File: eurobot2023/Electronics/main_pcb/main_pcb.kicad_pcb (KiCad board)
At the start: 2 copper layers, 103.1 x 93.2 mm, 51 parts, among them IC1 CD74HCT125M96, IC2 SN74LVC126ADR, J1 PI40HAT, J10 Conn_01x02_Male, J11 MagneticEncoder, J12 Conn_01x07_Male, J13 MagneticEncoder, J14 Conn_01x03_Male, J15 Conn_01x02_Male, J16 Conn_01x02_Male, J17 Conn_01x02_Male, J18 Conn_01x02_Male, J19 Conn_01x02_Male, J2 Conn_01x02_Male, J20 Conn_01x03_Male, J21 Conn_01x03_Male, J22 Conn_01x02_Male, J23 Conn_01x02_Male, J24 Conn_01x03_Male, J3 Conn_01x02_Male, J4 Conn_01x02_Male, J5 Conn_01x02_Male, J6 Conn_01x02_Male, J7 Conn_01x02_Male, J8 Conn_01x02_Male, J9 22-03-5035, P1 R-78Bxx-2.0, P2 Amazon 10A stepdown, Q1 2SK4017_Q_, Q2 2SK4017_Q_, Q3 2SK4017_Q_, Q4 2SK4017_Q_, Q5 2SK4017_Q_, Q6 2SK4017_Q_, U1 MCP2515-xSO, U2 TJA1049T, U3 PCA9306D, U4 Pololu_MAX14870, U5 PCA9685PW, U6 Pololu_MAX14870

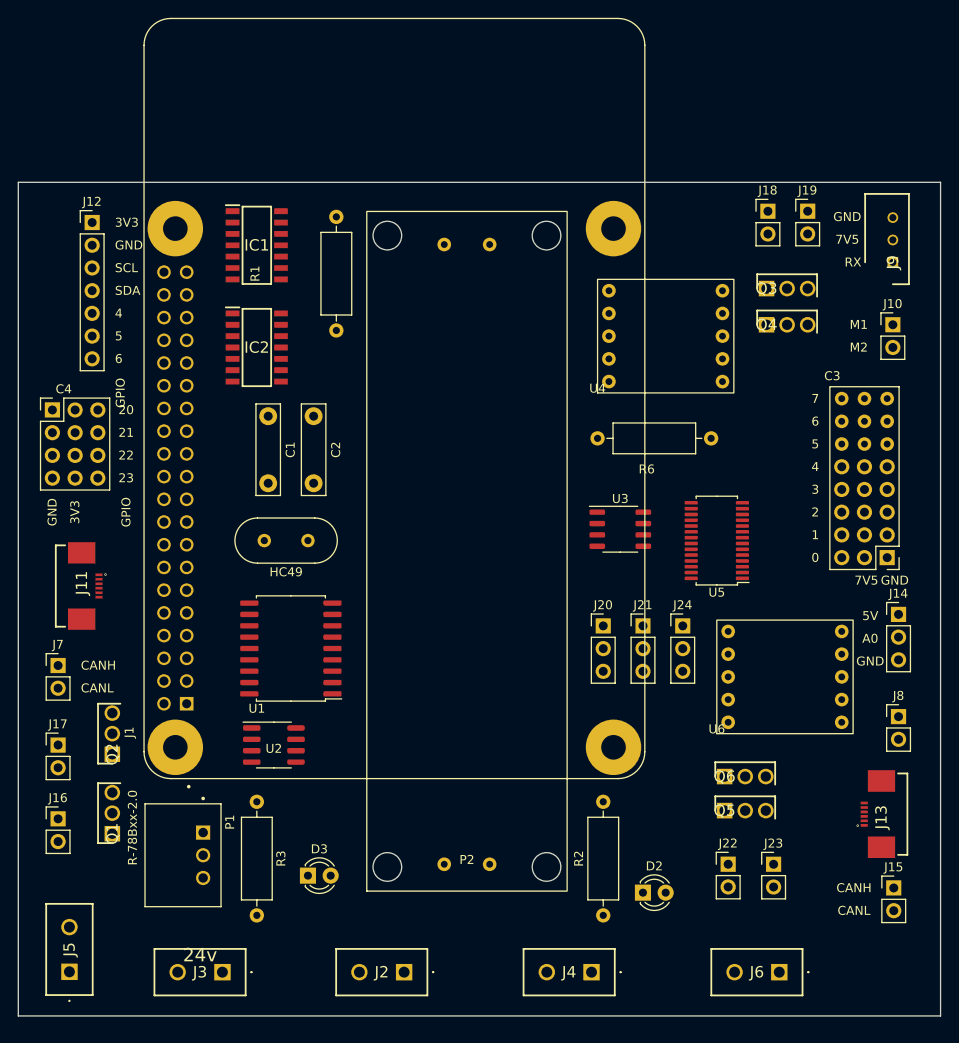
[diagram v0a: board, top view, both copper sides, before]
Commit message: Main PCB: update component placement.
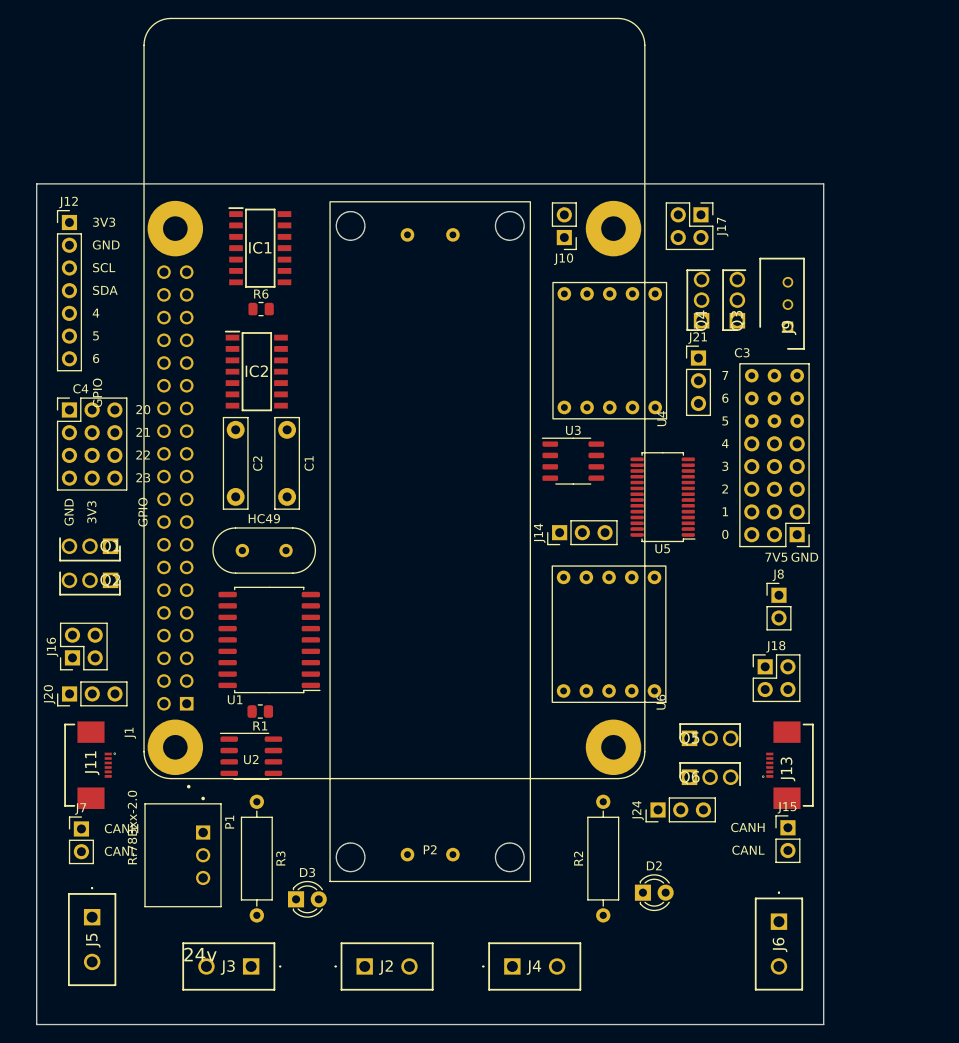
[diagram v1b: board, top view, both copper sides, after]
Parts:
- removed J19, J22, J23: Conn_01x02_Male, Connector_PinHeader_2.54mm:PinHeader_1x02_P2.54mm_Vertical
- J16, J17, J18: value Conn_01x02_Male -> Conn_02x02_Odd_Even; footprint Connector_PinHeader_2.54mm:PinHeader_1x02_P2.54mm_Vertical -> Connector_PinHeader_2.54mm:PinHeader_2x02_P2.54mm_Vertical
- R1, R6: footprint Resistor_THT:R_Axial_DIN0309_L9.0mm_D3.2mm_P12.70mm_Horizontal -> Resistor_SMD:R_0805_2012Metric
- moved J17 93.2 mm to (144.3, 59.5), turned to -90 degrees
- moved J20 60.2 mm to (73.7, 113.0), turned to 90 degrees
- moved R6 52.4 mm to (95.1, 70.0), turned to 0 degrees
- moved J18 50.9 mm to (151.5, 110.0)
- moved R1 43.5 mm to (95.0, 115.0), turned to 180 degrees
- moved J14 39.0 mm to (128.5, 95.0), turned to 90 degrees
- moved J10 38.0 mm to (129.0, 62.0), turned to 180 degrees
- moved Q1 32.1 mm to (78.3, 96.5), turned to 180 degrees
- moved J21 30.6 mm to (144.0, 75.5)
- moved J24 20.8 mm to (139.5, 126.0), turned to 90 degrees
- moved J11 20.1 mm to (77.5, 121.0)
- moved Q2 19.4 mm to (78.3, 100.3), turned to 180 degrees
- moved J8 19.0 mm to (153.0, 102.0)
- moved J7 18.5 mm to (75.0, 128.1)
- moved J16 18.1 mm to (74.0, 109.0), turned to 90 degrees
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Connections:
- J16 pad 1: Net-(J16-Pad1) -> Net-(J20-Pad2)
- J17 pad 1: Net-(J16-Pad1) -> Net-(J21-Pad2)
- J17 pad 2: Net-(J17-Pad2) -> Net-(Q3-Pad2)
- J18 pad 1: Net-(J18-Pad1) -> Net-(J24-Pad2)
- J18 pad 2: Net-(J18-Pad2) -> Net-(Q5-Pad2)
- J20 pad 2: Net-(J16-Pad1) -> Net-(J20-Pad2)
- J21 pad 2: Net-(J18-Pad1) -> Net-(J21-Pad2)
- J24 pad 2: Net-(J22-Pad1) -> Net-(J24-Pad2)
- Q2 pad 2: Net-(J17-Pad2) -> Net-(Q2-Pad2)
- Q3 pad 2: Net-(J18-Pad2) -> Net-(Q3-Pad2)
- Q4 pad 2: Net-(J19-Pad2) -> Net-(Q4-Pad2)
- Q5 pad 2: Net-(J22-Pad2) -> Net-(Q5-Pad2)
- Q6 pad 2: Net-(J23-Pad2) -> Net-(Q6-Pad2)
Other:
- board size 103.1 x 93.2 mm -> 88 x 94 mm
- board text removed: "5V"
- board text removed: "A0"
- board text removed: "M1"
- board text removed: "M2"
- board text removed: "RX"
